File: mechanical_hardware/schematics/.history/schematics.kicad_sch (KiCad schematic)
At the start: 5 parts, among them U1:5,1V CRE1S0305S3C, U2:5V CRE1S0305S3C, U3:12V CRE1S0305S3C

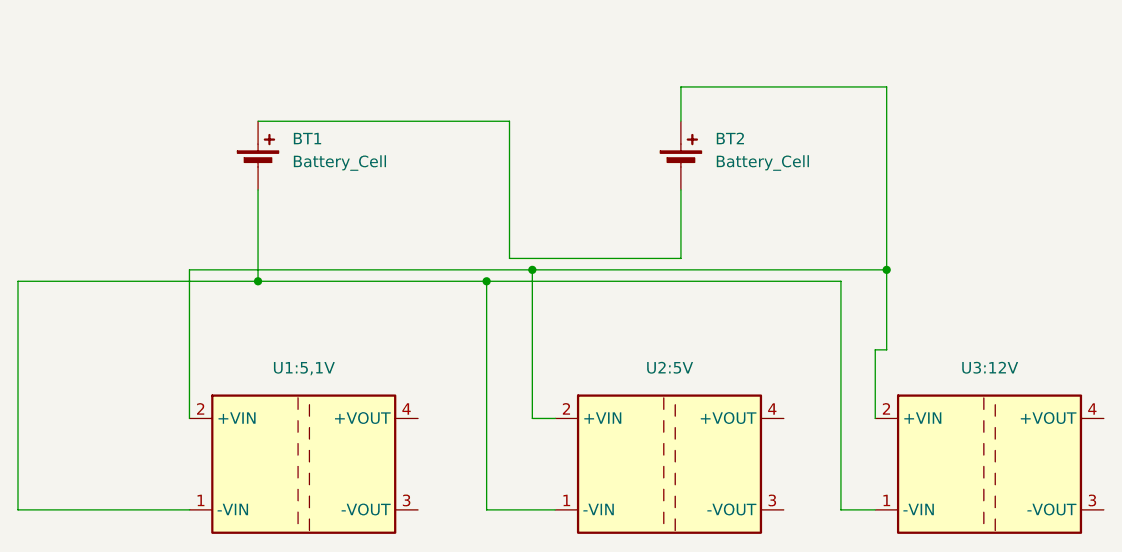
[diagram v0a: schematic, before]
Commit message: schematics backup
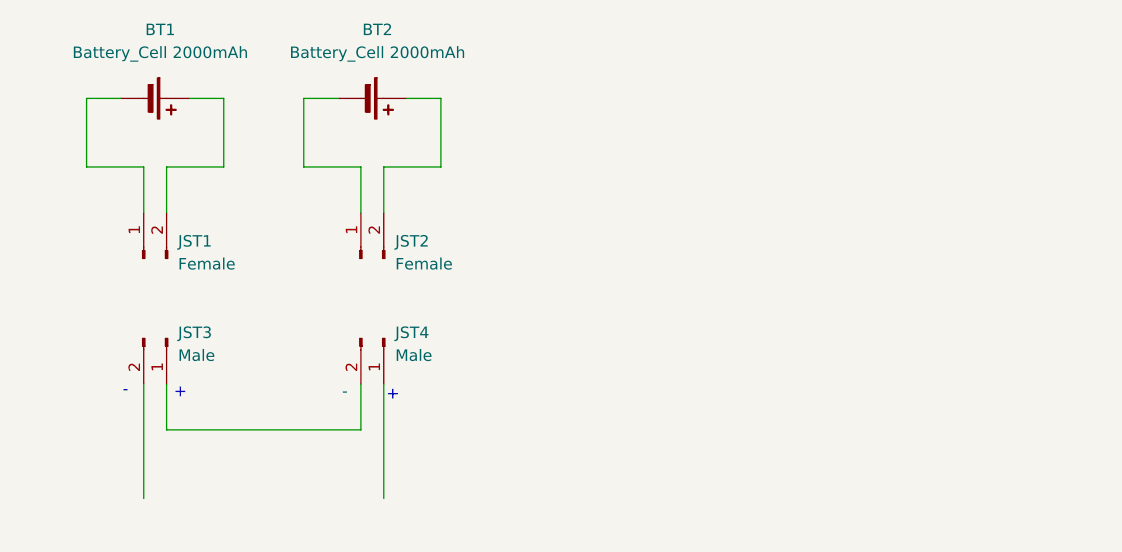
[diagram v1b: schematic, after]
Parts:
- removed U1:5,1V, U2:5V, U3:12V: CRE1S0305S3C, Converter_DCDC:Converter_DCDC_Murata_CRE1xxxxxx3C_THT, symbol Regulator_Switching:CRE1S0305S3C
- added JST1, JST2: Female, symbol Connector:Conn_01x02_Pin
- added JST3, JST4: Male, symbol Connector:Conn_01x02_Pin
- BT1, BT2: value Battery_Cell -> Battery_Cell 2000mAh
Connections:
- net at BT2.1 (+): now also JST2.2 (Pin_2)
- net at BT2.2 (-): now also JST2.1 (Pin_1); no longer BT1.1 (+)
- net at BT1.2 (-): now also JST1.1 (Pin_1)
- new net: BT1.1 (+), JST1.2 (Pin_2)
- new net: JST3.1 (Pin_1), JST4.2 (Pin_2)
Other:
- note added: "+"
- note added: "-"
